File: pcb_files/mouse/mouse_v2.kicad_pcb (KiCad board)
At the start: 2 copper layers, 94.7 x 94.9 mm, 72 parts, among them J2 BT_Conn, J4 I2C_Conn, M1 Motor_DC, M2 Motor_DC, M3 CASTER_BALL, Q0 Q_Photo_NPN, Q1 Q_Photo_NPN, Q2 Q_Photo_NPN, Q3 Q_Photo_NPN, SW1 TL3315NF160Q, SW2 TL3315NF160Q, T0 Q_NMOS_DGS, T1 Q_NMOS_DGS, T2 Q_NMOS_DGS, T3 Q_NMOS_DGS, U1 Teensy3.2, U2 SN754410NE, U3 LM1084-5.0, U4 Encoder_3081, U5 Encoder_3081

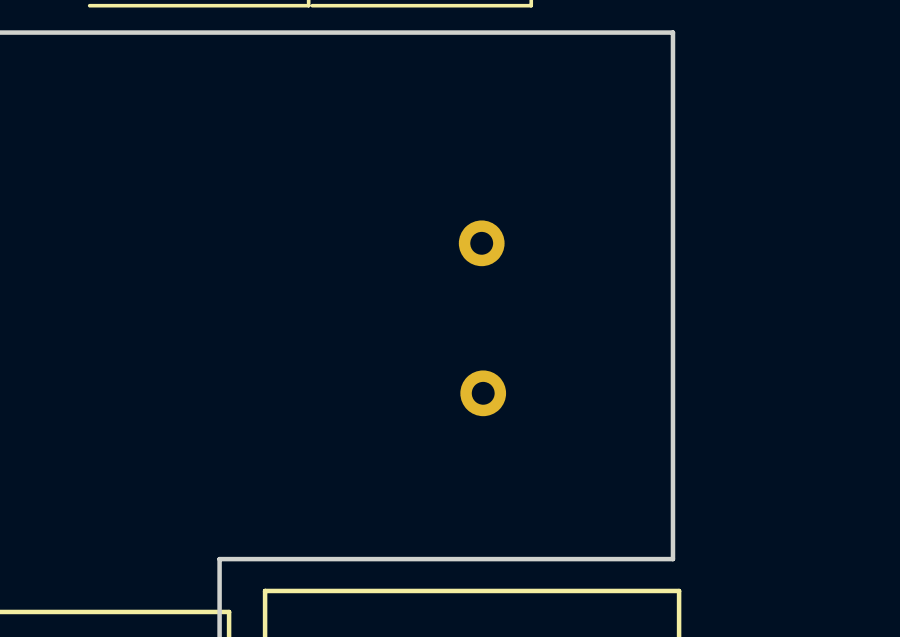
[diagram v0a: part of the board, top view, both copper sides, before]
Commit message: Start of v3.0
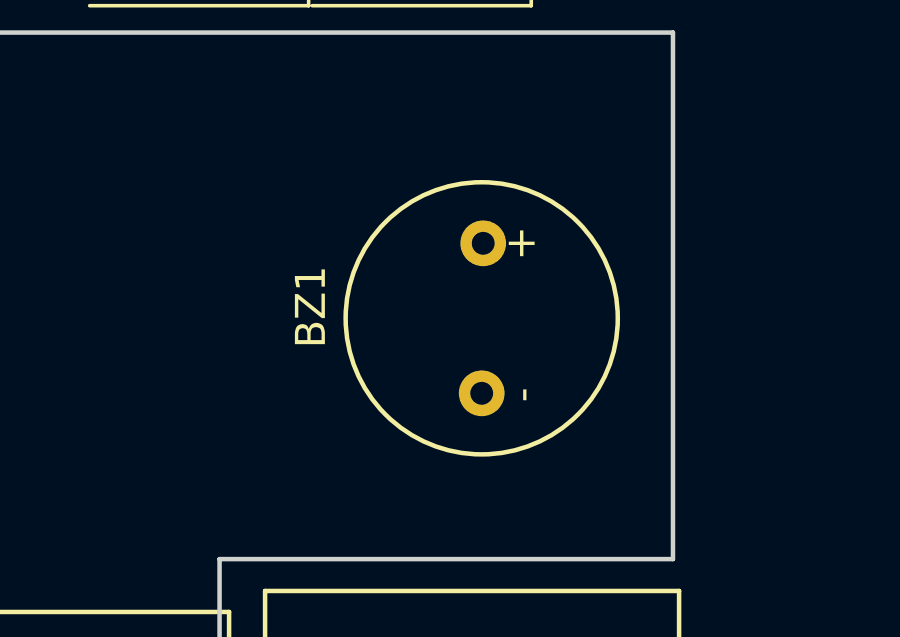
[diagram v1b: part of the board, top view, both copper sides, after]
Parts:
- BZ1: moved to F.Cu
- turned BZ1 to 90 degrees
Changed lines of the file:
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@@
   (general
     (thickness 1.6)
-    (drawings 43)
+    (drawings 41)
     (tracks 0)
     (zones 0)
@@
     (pad "" np_thru_hole circle (at -26.75 -9 180) (size 2.1844 2.1844) (drill 2.1844) (layers *.Cu *.Mask))
   )
-  (module "misc:9x5.5mm Buzzer" (layer B.Cu)
-    (at 200.9648 64.1858 270)
-    (fp_text reference BZ1 (at 0.381 5.6896 270) (layer B.SilkS)
-      (effects (font (size 1 1) (thickness 0.15)) (justify mirror))
+  (module "misc:9x5.5mm Buzzer" (layer F.Cu)
+    (at 200.9648 64.1858 90)
+    (fp_text reference BZ1 (at 0.381 -5.6896 90) (layer F.SilkS)
+      (effects (font (size 1 1) (thickness 0.15)))
     )
-    (fp_text value Buzzer (at -0.05 -6.8 270) (layer B.Fab)
-      (effects (font (size 1 1) (thickness 0.15)) (justify mirror))
+    (fp_text value Buzzer (at -0.05 6.8 90) (layer F.Fab)
+      (effects (font (size 1 1) (thickness 0.15)))
     )
-    (fp_circle (center 0 0) (end 4.4 1.1) (layer B.SilkS) (width 0.15))
-    (fp_text user - (at -2.55 -1.35 270) (layer B.SilkS)
-      (effects (font (size 1 1) (thickness 0.15)) (justify mirror))
+    (fp_circle (center 0 0) (end 4.4 -1.1) (layer F.SilkS) (width 0.15))
+    (fp_text user - (at -2.55 1.35 90) (layer F.SilkS)
+      (effects (font (size 1 1) (thickness 0.15)))
     )
-    (fp_text user + (at 2.5 -1.3 270) (layer B.SilkS)
-      (effects (font (size 1 1) (thickness 0.15)) (justify mirror))
+    (fp_text user + (at 2.5 1.3 90) (layer F.SilkS)
+      (effects (font (size 1 1) (thickness 0.15)))
     )
-    (pad 2 thru_hole circle (at -2.5 0 270) (size 1.524 1.524) (drill 0.762) (layers *.Cu *.Mask)
+    (pad 2 thru_hole circle (at -2.5 0 90) (size 1.524 1.524) (drill 0.762) (layers *.Cu *.Mask)
       (net 2 /GND))
-    (pad 1 thru_hole circle (at 2.5 -0.05 270) (size 1.524 1.524) (drill 0.762) (layers *.Cu *.Mask)
+    (pad 1 thru_hole circle (at 2.5 0.05 90) (size 1.524 1.524) (drill 0.762) (layers *.Cu *.Mask)
       (net 50 "Net-(BZ1-Pad1)"))
   )
@@
   (gr_line (start 207.3402 102.4128) (end 192.2272 102.4128) (layer Edge.Cuts) (width 0.15))
   (gr_line (start 112.5982 102.1588) (end 127.7112 102.1588) (layer Edge.Cuts) (width 0.15))
-  (dimension 10.9982 (width 0.3) (layer F.SilkS)
-    (gr_text "10.998 mm" (at 218.508 100.4951 90) (layer F.SilkS)
-      (effects (font (size 1.5 1.5) (thickness 0.3)))
-    )
-    (feature1 (pts (xy 144.9832 94.996) (xy 216.994421 94.996)))
-    (feature2 (pts (xy 144.9832 105.9942) (xy 216.994421 105.9942)))
-    (crossbar (pts (xy 216.408 105.9942) (xy 216.408 94.996)))
-    (arrow1a (pts (xy 216.408 94.996) (xy 216.994421 96.122504)))
-    (arrow1b (pts (xy 216.408 94.996) (xy 215.821579 96.122504)))
-    (arrow2a (pts (xy 216.408 105.9942) (xy 216.994421 104.867696)))
-    (arrow2b (pts (xy 216.408 105.9942) (xy 215.821579 104.867696)))
-  )
-  (dimension 26.823855 (width 0.3) (layer F.SilkS)
-    (gr_text "26.824 mm" (at 128.255363 118.054665 359.4031905) (layer F.SilkS)
-      (effects (font (size 1.5 1.5) (thickness 0.3)))
-    )
-    (feature1 (pts (xy 142.0114 85.09) (xy 141.682328 116.680868)))
-    (feature2 (pts (xy 115.189 84.8106) (xy 114.859928 116.401468)))
-    (crossbar (pts (xy 114.866037 115.815079) (xy 141.688437 116.094479)))
-    (arrow1a (pts (xy 141.688437 116.094479) (xy 140.555886 116.669134)))
-    (arrow1b (pts (xy 141.688437 116.094479) (xy 140.568103 115.496356)))
-    (arrow2a (pts (xy 114.866037 115.815079) (xy 115.986371 116.413202)))
-    (arrow2b (pts (xy 114.866037 115.815079) (xy 115.998588 115.240424)))
-  )
   (gr_text v2.0 (at 182.1942 55.9054 180) (layer B.SilkS)
     (effects (font (size 1.5 1.5) (thickness 0.3)) (justify mirror))
